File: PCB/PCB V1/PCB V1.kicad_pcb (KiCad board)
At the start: 2 copper layers, 55 parts, among them J1 Screw_Terminal_01x03, J2 Screw_Terminal_01x03, J3 USB_B, J4 Conn_01x02_Pin, K1 Relay_SPDT, K2 Relay_SPDT, Q1 S8050, Q2 S8050, Q3 S8050, SW1 On/Off, SW2 SW_Push, SW3 SW_Push, U1 LM317_TO-220, U2 LM317_TO-220

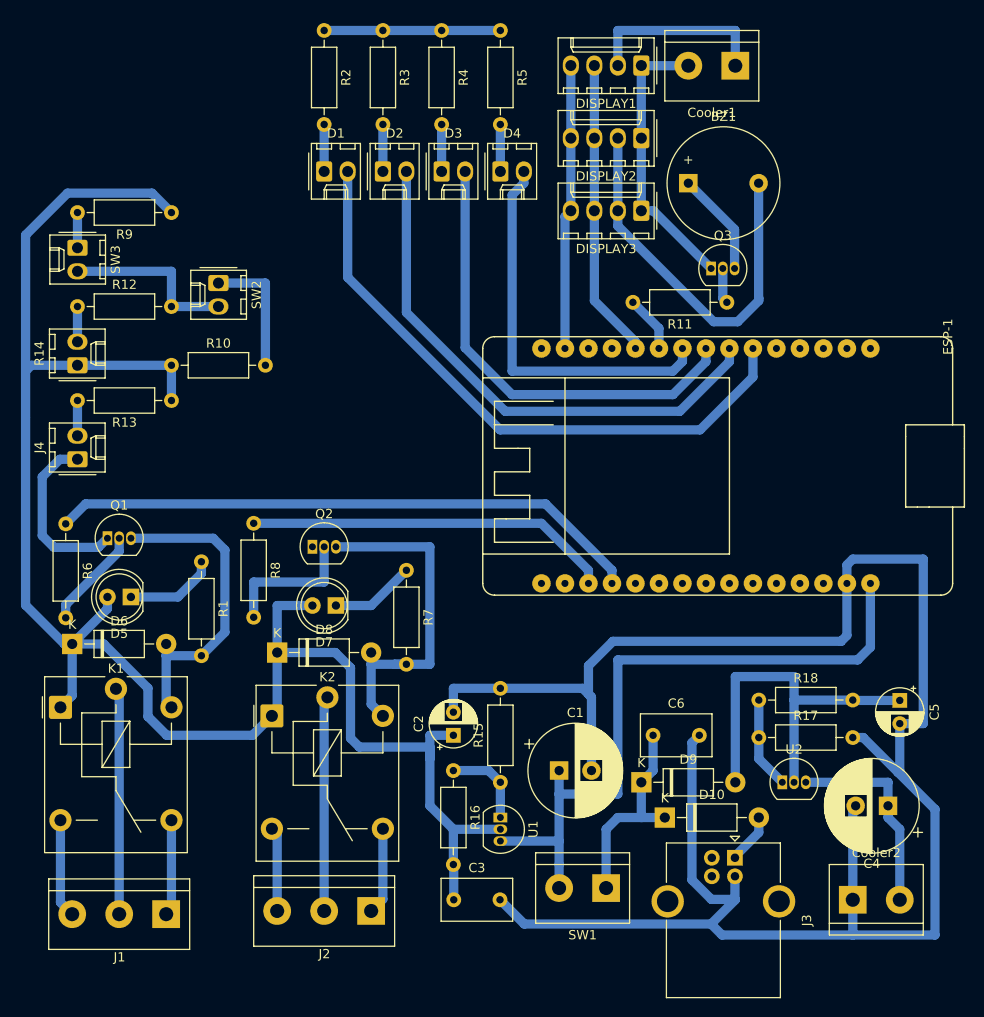
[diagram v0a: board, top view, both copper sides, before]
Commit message: .
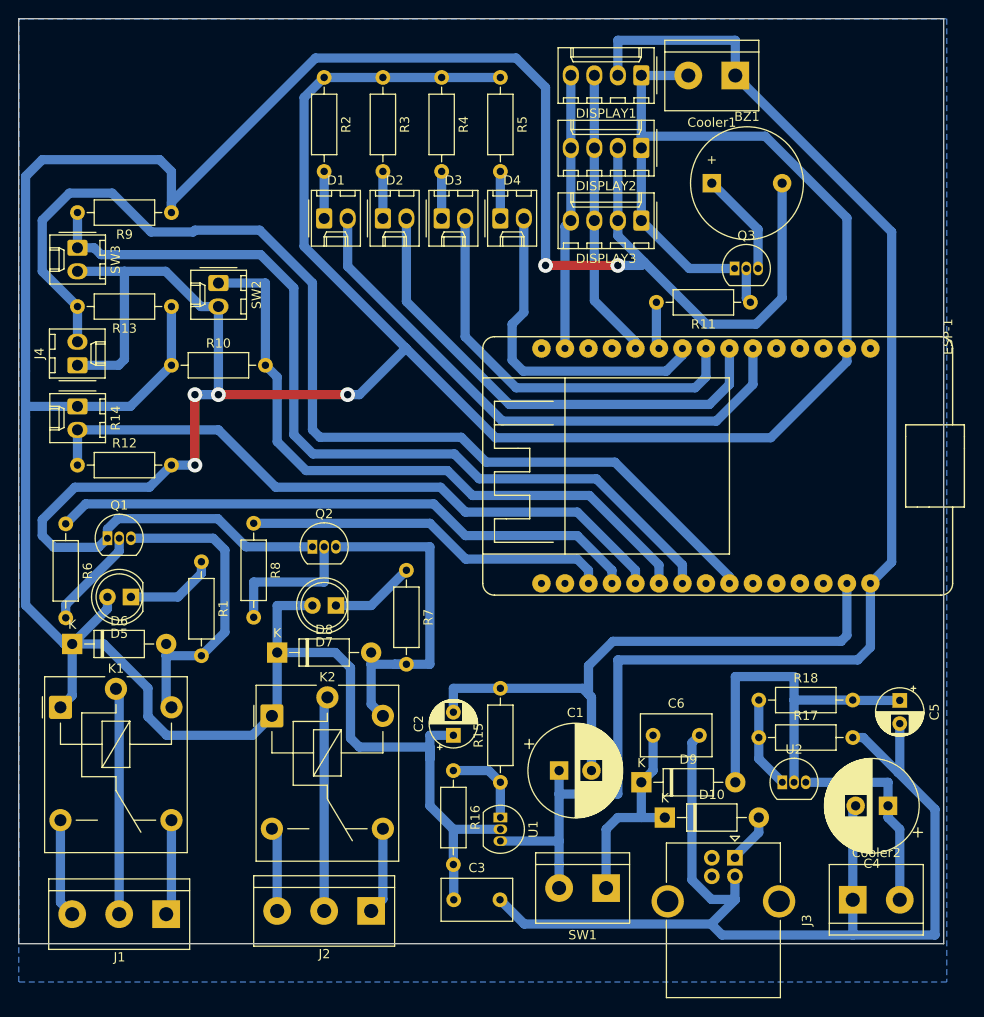
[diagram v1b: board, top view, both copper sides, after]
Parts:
- moved R12 17.1 mm to (188.0, 63.5)
- moved J4 10.2 mm to (188.0, 52.7)
- moved R13 10.2 mm to (198.1, 46.4)
- moved D1 5.08 mm to (214.6, 36.8)
- moved D2 5.08 mm to (221.0, 36.8)
- moved D3 5.08 mm to (227.3, 36.8)
- moved D4 5.08 mm to (233.7, 36.8)
- moved R2 5.08 mm to (214.6, 21.6)
- moved R3 5.08 mm to (221.0, 21.6)
- moved R4 5.08 mm to (227.3, 21.6)
- moved R5 5.08 mm to (233.7, 21.6)
- moved R14 4.45 mm to (188.0, 57.1), turned to -90 degrees
- moved BZ1 2.54 mm to (256.5, 33.0)
- moved Q3 2.54 mm to (259.0, 42.2)
- moved R11 2.54 mm to (260.7, 45.9)
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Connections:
- ESP-1 pad 10: unconnected-(ESP-1-IO32-Pad10) -> BOTON-A
- ESP-1 pad 16: BOTON-A -> unconnected-(ESP-1-IO23-Pad16)
- ESP-1 pad 26: PUERTA -> unconnected-(ESP-1-IO4-Pad26)
- ESP-1 pad 7: BOTON-B -> PUERTA
- ESP-1 pad 9: unconnected-(ESP-1-IO33-Pad9) -> BOTON-B
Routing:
- net GND: track 304.6 -> 496.3 mm, vias 0 -> 4
- net PUERTA: track 3.81 -> 117.6 mm
- net +3.3V: track 239.1 -> 334.1 mm, vias 0 -> 2
- net BOTON-B: track 3.81 -> 94.7 mm
- net LDR: track 3.81 -> 71.8 mm
- net +5V: track 95.0 -> 157.8 mm
- net BOTON-A: track 14.0 -> 71.5 mm
- net LED-B2: track 42.4 -> 36.2 mm
- net LED-A1: track 67.5 -> 61.5 mm
- net LED-A2: track 50.1 -> 44.7 mm
- net LED-B1: track 58.2 -> 53.3 mm
- net SDA: track 32.4 -> 31.4 mm
- net SCL: track 30.9 -> 29.8 mm
- net BUZZER: track 6.16 -> 5.10 mm
- added copper zone on B.Cu, net GND
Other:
- board outline added: 100 x 100 mm
